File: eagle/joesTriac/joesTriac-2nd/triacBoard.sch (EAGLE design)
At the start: 16 parts, among them X1 1751316, X2 1751248

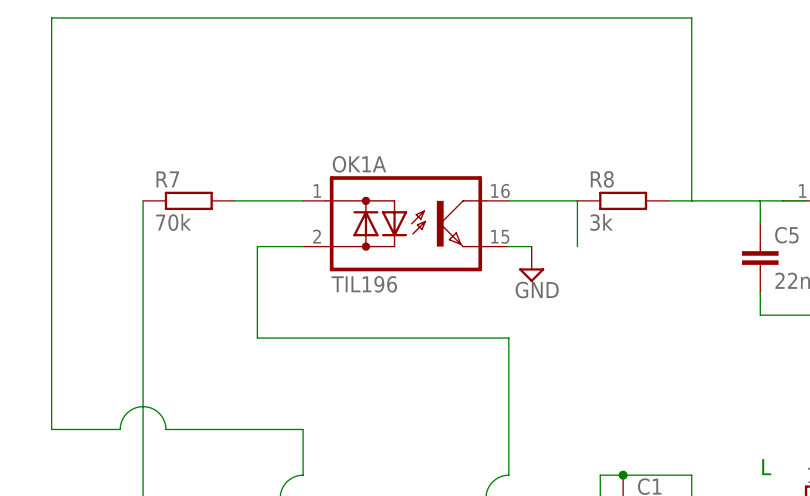
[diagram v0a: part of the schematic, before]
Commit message: candidate for release
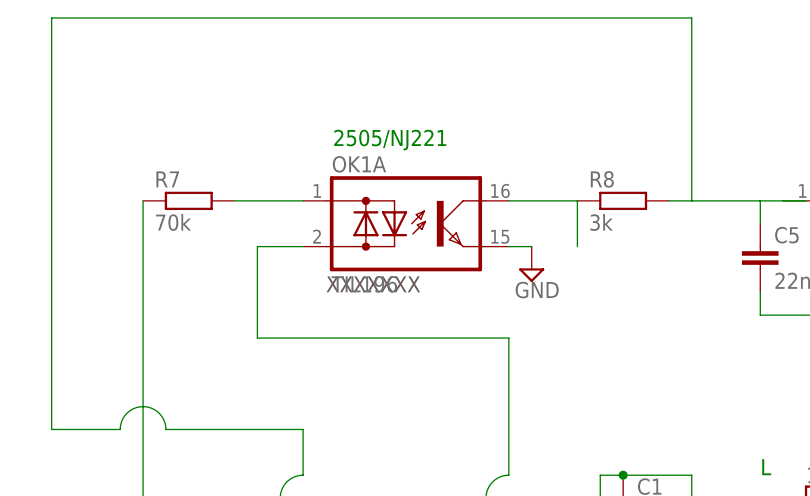
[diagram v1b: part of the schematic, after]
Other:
- note added: "2505/NJ221"
- note added: "XXXXXXX"
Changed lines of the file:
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@@
 <text x="-93.98" y="60.96" size="1.778" layer="91">=====</text>
 <text x="-88.9" y="60.96" size="1.778" layer="91">=====</text>
+<text x="-2.54" y="111.76" size="1.778" layer="92">XXXXXXX</text>
+<text x="-1.778" y="128.016" size="1.778" layer="91">2505/NJ221</text>
 </plain>
 <instances>
